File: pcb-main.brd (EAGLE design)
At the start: 100 x 80 mm, 80 parts, among them U1 IH1224DH, U2 RS3-1215D, U3 56DP30-GAIN

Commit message: Add component value for LT3032-12 module
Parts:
- U4: value (none) -> F-LT3032-12
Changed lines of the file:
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@@
 <element name="U1" library="regulators-switch-mode" package="SIP7" value="IH1224DH" x="44" y="77"/>
 <element name="U2" library="regulators-switch-mode" package="SIP8" value="RS3-1215D" x="24" y="67.5" rot="R270"/>
-<element name="U4" library="module-footprints" package="F-DIP8-HEATSINK" value="" x="44" y="61" rot="R270"/>
+<element name="U4" library="module-footprints" package="F-DIP8-HEATSINK" value="F-LT3032-12" x="44" y="61" rot="R270"/>
 <element name="L1" library="inductors" package="BL01RN1A" value="BL01RN1A1F1J" x="6" y="58" rot="R90">
 <attribute name="MOUSER" value="81-BL01RN1A1F1J" x="6" y="58" size="1.778" layer="27" rot="R90" display="off"/>

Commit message: Change DC Connector
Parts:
- XS4: value 712RA -> 722RA
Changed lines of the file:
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@@
 <elements>
 <element name="E$1" library="enclosure" package="B*-080" value="" x="0" y="0"/>
-<element name="XS4" library="connectors" package="SWITCHCRAFT-L712RA" value="712RA" x="10" y="80" rot="R270">
+<element name="XS4" library="connectors" package="SWITCHCRAFT-L712RA" value="722RA" x="10" y="80" rot="R270">
 <attribute name="MOUSER" value="502-722RA" x="10" y="80" size="1.778" layer="27" rot="R270" display="off"/>
 </element>

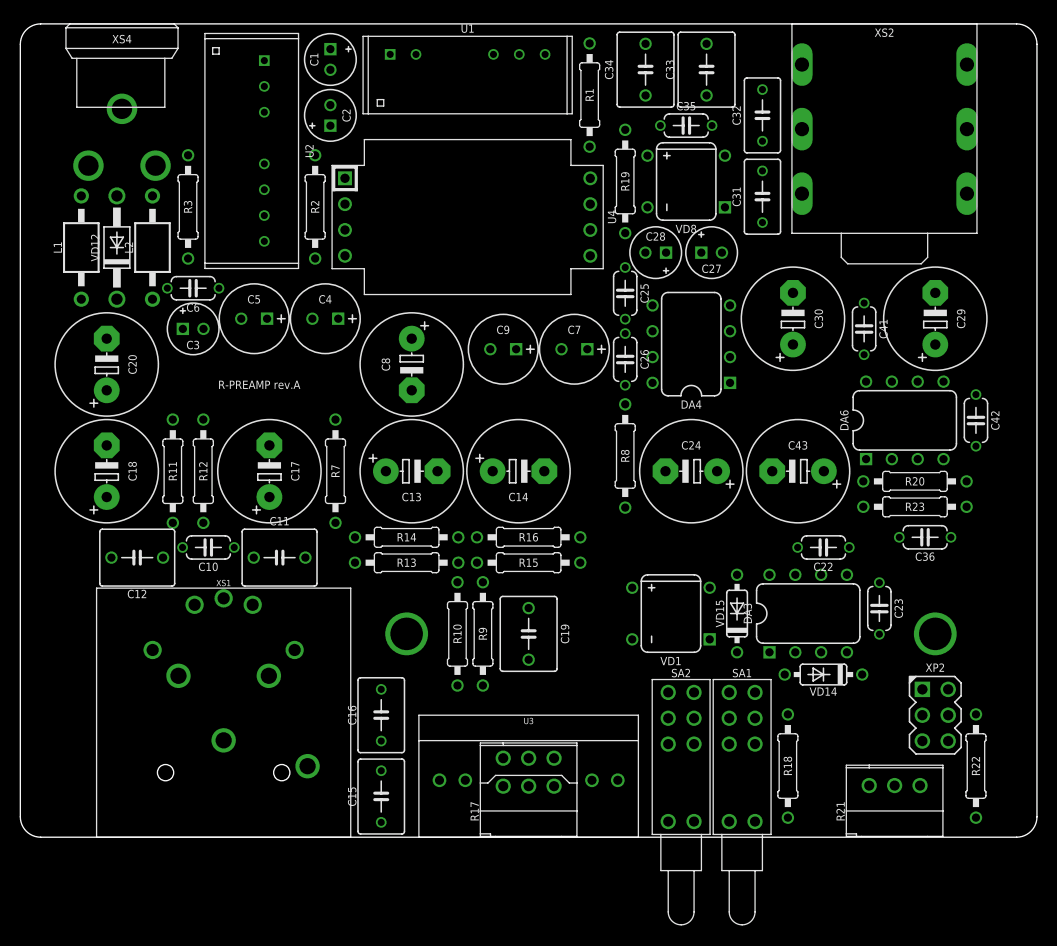
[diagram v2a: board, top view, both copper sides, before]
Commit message: PCB Routing
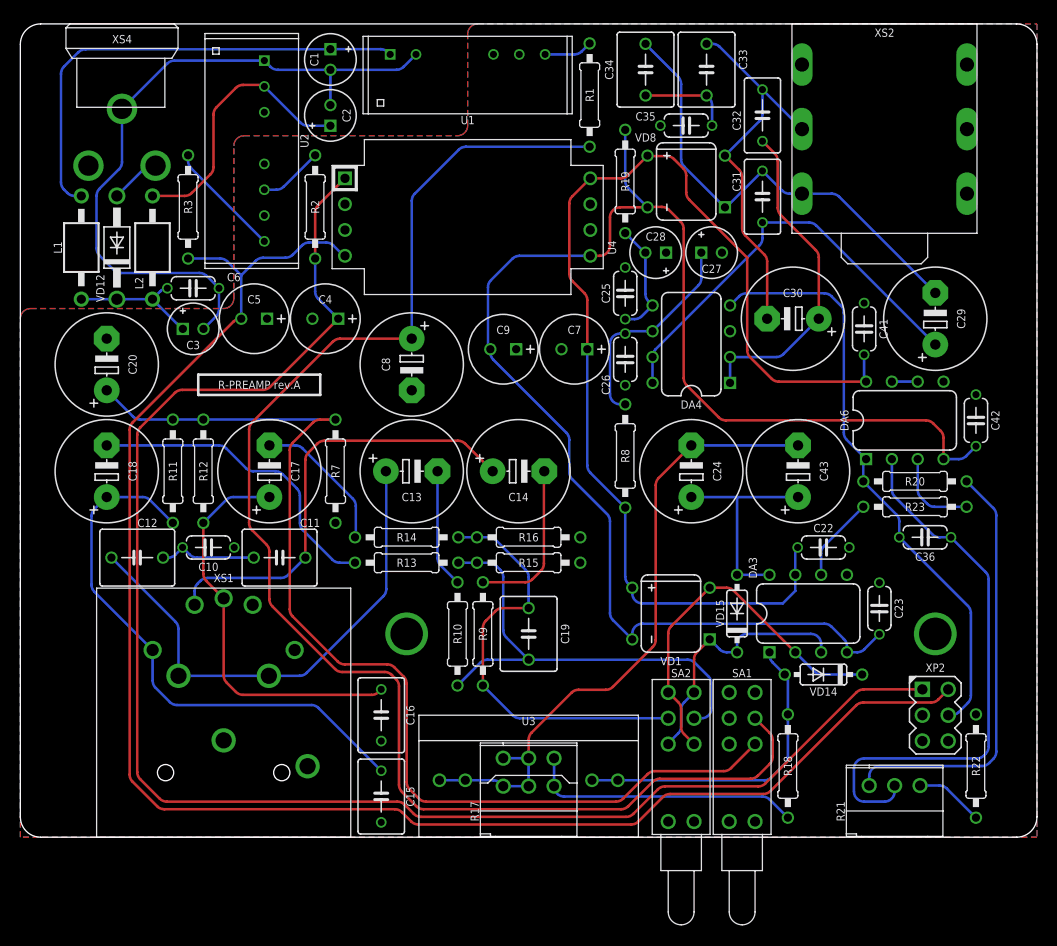
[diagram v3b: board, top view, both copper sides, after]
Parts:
- turned C24 to 90 degrees
- turned C30 to 180 degrees
- turned C43 to 90 degrees
- turned R23 to 180 degrees
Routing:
- net -15V: track 0.00 -> 159.2 mm
- net +15V: track 0.00 -> 157.6 mm
- net -12V: track 0.00 -> 150.1 mm
- net +48V: track 0.00 -> 141.2 mm
- net +12V: track 0.00 -> 111.9 mm
- net N$23: track 0.00 -> 106.9 mm
- net CHASSIS: track 0.00 -> 68.1 mm
- net N$21: track 0.00 -> 63.8 mm
- net N$40: track 0.00 -> 58.6 mm
- net N$37: track 0.00 -> 54.9 mm
- net N$13: track 0.00 -> 54.8 mm
- net N$11: track 0.00 -> 50.0 mm
- net N$3: track 0.00 -> 47.0 mm
- net N$29: track 0.00 -> 46.2 mm
- net N$33: track 0.00 -> 45.8 mm
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- added copper zone on layer 1, net GND
- added copper zone on layer 16, net GND

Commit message: Change 20R -> 22R
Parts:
- R19, R8: value 20R(TH) -> 22R(TH)
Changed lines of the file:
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@@
 <element name="C27" library="capacitors-electrolytic" package="E2-5" value="47U/35V" x="68" y="57.5"/>
 <element name="C28" library="capacitors-electrolytic" package="E2-5" value="47U/35V" x="62.5" y="57.5" rot="R180"/>
-<element name="R8" library="resistors" package="R-0207/10" value="20R(TH)" x="59.5" y="37.5" rot="R270"/>
-<element name="R19" library="resistors" package="R-0207/10" value="20R(TH)" x="59.5" y="64.5" rot="R90"/>
+<element name="R8" library="resistors" package="R-0207/10" value="22R(TH)" x="59.5" y="37.5" rot="R270"/>
+<element name="R19" library="resistors" package="R-0207/10" value="22R(TH)" x="59.5" y="64.5" rot="R90"/>
 <element name="C29" library="capacitors-electrolytic" package="E5-10,5" value="47U/35V(NP)" x="90" y="51" rot="R90"/>
 <element name="C30" library="capacitors-electrolytic" package="E5-10,5" value="47U/35V(NP)" x="76" y="51" rot="R180"/>
